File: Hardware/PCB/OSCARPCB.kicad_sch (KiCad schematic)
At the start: 10 parts, among them J1 CP2102 IN, J2 Stepper Motor OUT, J3 DC Motors OUT, J4 Servo OUT, J5 Power Input, U1 L293D, U2 ESP32-DevKitC

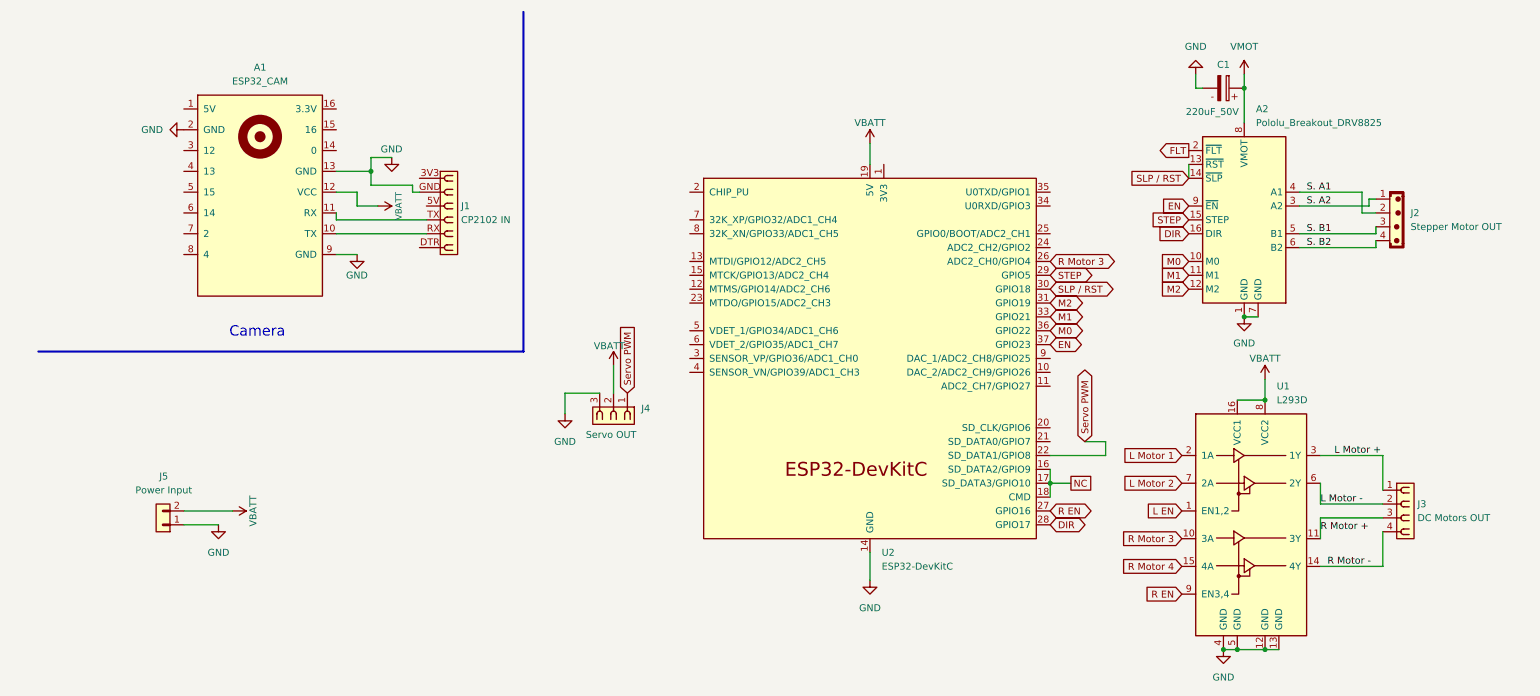
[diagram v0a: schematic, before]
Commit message: PCB V1
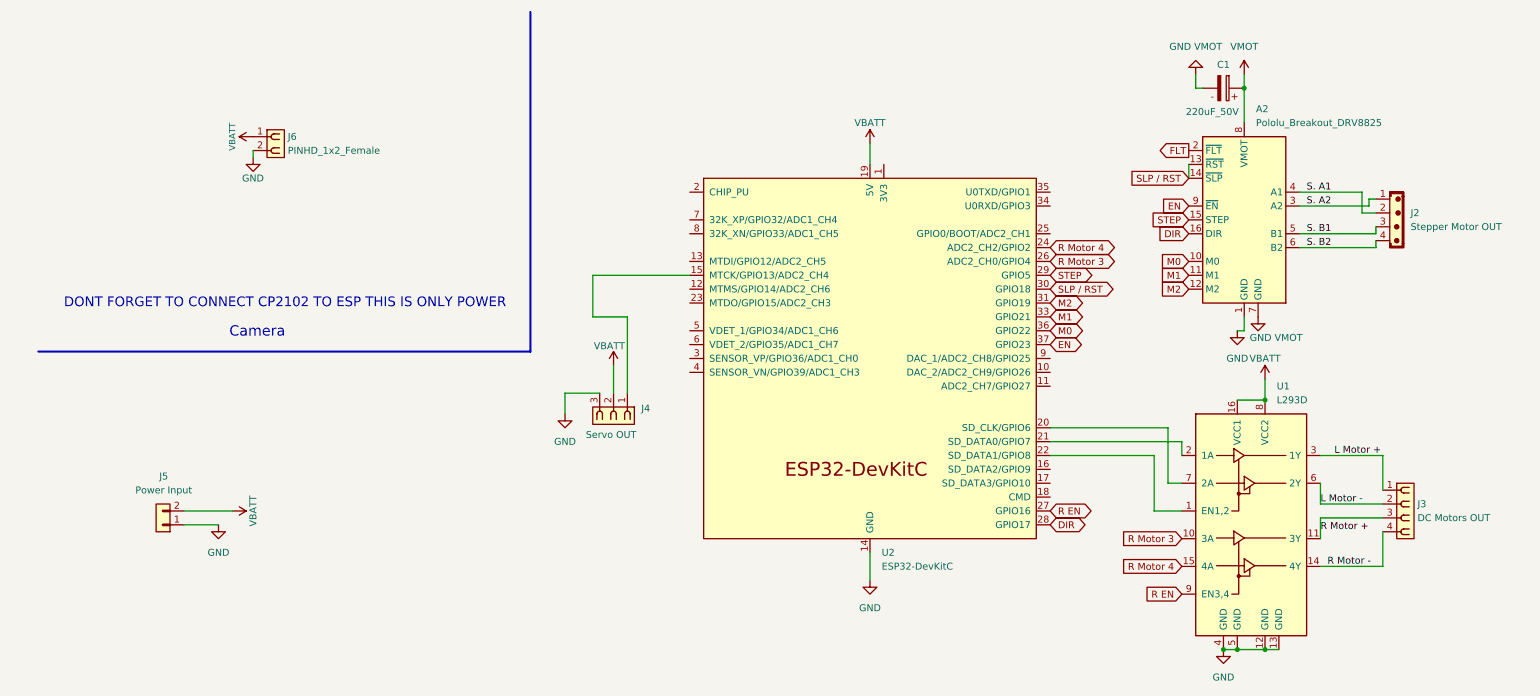
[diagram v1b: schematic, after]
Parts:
- removed A1: ESP32_CAM, PCM_SL_Development_Boards:ESP32-CAM, symbol PCM_SL_Development_Board:ESP32_CAM
- removed J1: CP2102 IN, Connector_PinSocket_2.54mm:PinSocket_1x06_P2.54mm_Vertical, symbol PCM_SL_Pin_Headers:PINHD_1x6_Female
- added J6: PINHD_1x2_Female, Connector_PinSocket_2.54mm:PinSocket_1x02_P2.54mm_Vertical, symbol PCM_SL_Pin_Headers:PINHD_1x2_Female
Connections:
- net L Motor 1 is gone; now on an unnamed net: U1.2 (1A)
- net L Motor 2 is gone; now on an unnamed net: U1.7 (2A)
- net GND: now also J6.2; no longer A2.7 (GND), C1.2
- net R Motor 4: now also U2.24 (ADC2_CH2/GPIO2)
- net VBATT: now also J6.1
- net at U2.15 (MTCK/GPIO13/ADC2_CH4): now also J4.1
- net L EN: no longer names the net of U1.1 (EN1,2)
- net L EN: now also U2.22 (SD_DATA1/GPIO8)
- removed net NC: U2.16 (SD_DATA2/GPIO9), U2.17 (SD_DATA3/GPIO10), U2.18 (CMD)
- removed net Servo PWM: J4.1, U2.22 (SD_DATA1/GPIO8)
- new net GND VMOT: A2.7 (GND), C1.2
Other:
- note added: "DONT FORGET TO CONNECT CP2102 TO ESP THIS IS ONLY POWER"
